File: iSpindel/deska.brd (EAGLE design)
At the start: 49.2 x 29.2 mm, 21 parts

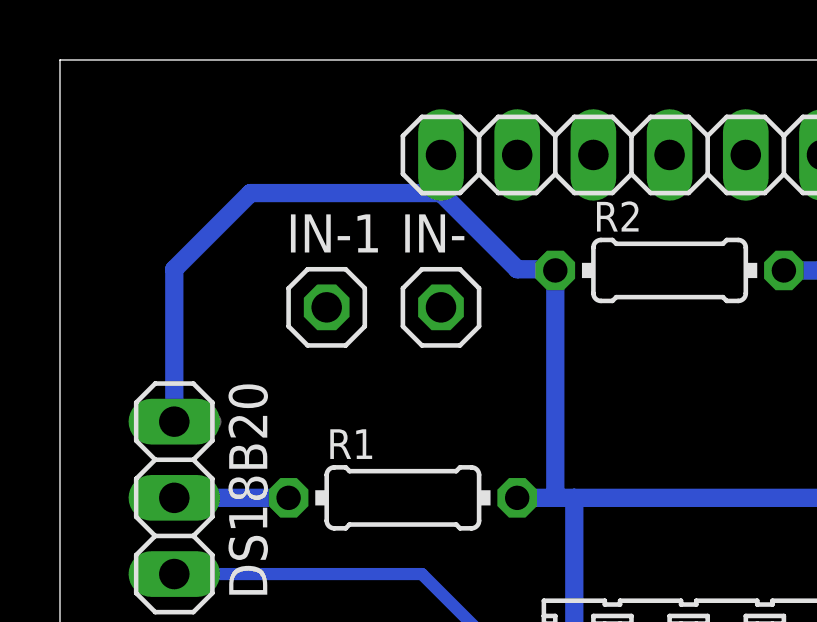
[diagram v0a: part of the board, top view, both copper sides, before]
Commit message: uprava desky
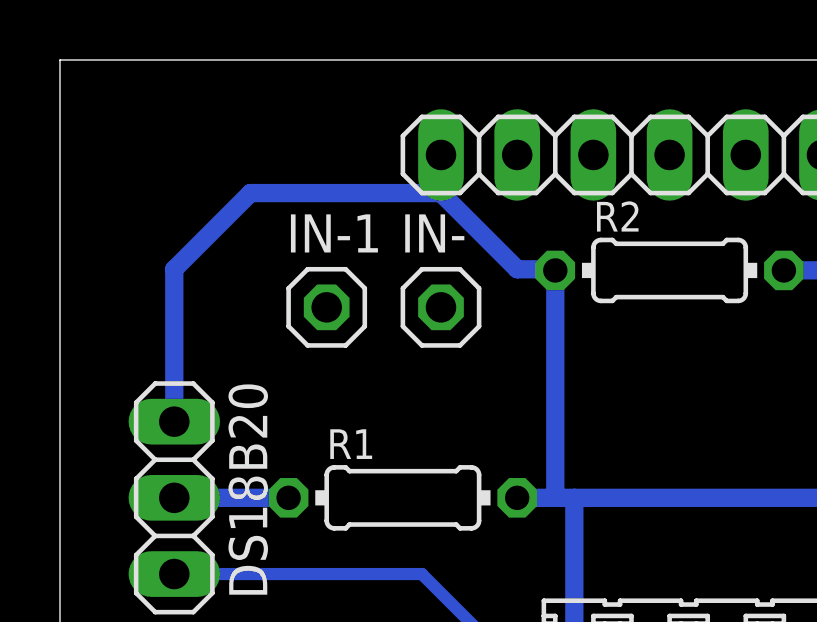
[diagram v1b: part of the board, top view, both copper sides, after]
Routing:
- net +3V3: track 65.3 -> 64.0 mm, vias 1 -> 0
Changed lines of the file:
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@@
 <?xml version="1.0" encoding="utf-8"?>
 <!DOCTYPE eagle SYSTEM "eagle.dtd">
-<eagle version="7.7.0">
+<eagle version="9.1.3">
 <drawing>
 <settings>
 <setting alwaysvectorfont="no"/>
+<setting keepoldvectorfont="yes"/>
 <setting verticaltext="up"/>
 </settings>
@@
 <param name="dpMaxLengthDifference" value="10mm"/>
 <param name="dpGapFactor" value="2.5"/>
-<param name="checkGrid" value="0"/>
 <param name="checkAngle" value="0"/>
 <param name="checkFont" value="1"/>
 <param name="checkRestrict" value="1"/>
+<param name="checkStop" value="0"/>
+<param name="checkValues" value="0"/>
+<param name="checkNames" value="1"/>
+<param name="checkWireStubs" value="1"/>
+<param name="checkPolygonWidth" value="0"/>
 <param name="useDiameter" value="13"/>
 <param name="maxErrors" value="50"/>
@@
 <element name="IN+3" library="pinhead" package="1X01" value="" x="38.1" y="12.065"/>
 <element name="SL1" library="con-amp-quick" package="05P" value="" x="22.225" y="13.335" rot="R180">
+<attribute name="MF" value="" x="22.225" y="13.335" size="1.778" layer="27" rot="R180" display="off"/>
 <attribute name="MPN" value="" x="22.225" y="13.335" size="1.778" layer="27" rot="R180" display="off"/>
+<attribute name="OC_FARNELL" value="unknown" x="22.225" y="13.335" size="1.778" layer="27" rot="R180" display="off"/>
 <attribute name="OC_NEWARK" value="unknown" x="22.225" y="13.335" size="1.778" layer="27" rot="R180" display="off"/>
-<attribute name="OC_FARNELL" value="unknown" x="22.225" y="13.335" size="1.778" layer="27" rot="R180" display="off"/>
-<attribute name="MF" value="" x="22.225" y="13.335" size="1.778" layer="27" rot="R180" display="off"/>
 </element>
 <element name="IN+4" library="pinhead" package="1X01" value="" x="38.1" y="24.765"/>
@@
 <contactref element="R1" pad="2"/>
 <wire x1="12.7" y1="30.48" x2="12.7" y2="29.21" width="0.6096" layer="16"/>
-<wire x1="12.7" y1="29.21" x2="15.24" y2="26.67" width="0.6096" layer="16"/>
-<wire x1="15.24" y1="26.67" x2="16.47" y2="26.67" width="0.6096" layer="16"/>
-<wire x1="16.47" y1="26.67" x2="16.51" y2="26.63" width="0.6096" layer="1"/>
-<wire x1="3.81" y1="21.59" x2="5.08" y2="21.59" width="0.6096" layer="1"/>
 <wire x1="12.7" y1="29.21" x2="6.35" y2="29.21" width="0.6096" layer="16"/>
 <wire x1="6.35" y1="29.21" x2="3.81" y2="26.67" width="0.6096" layer="16"/>
 <wire x1="3.81" y1="26.67" x2="3.81" y2="21.59" width="0.6096" layer="16"/>
-<via x="16.47" y="26.67" extent="1-16" drill="0.6" shape="square"/>
 <contactref element="SL1" pad="5"/>
 <wire x1="15.24" y1="19.05" x2="16.51" y2="19.05" width="0.6096" layer="16"/>
@@
 <wire x1="27.305" y1="19.05" x2="17.145" y2="19.05" width="0.6096" layer="16"/>
 <wire x1="29.21" y1="12.7" x2="30.48" y2="11.43" width="0.6096" layer="16"/>
+<wire x1="16.51" y1="26.63" x2="16.47" y2="26.67" width="0.6096" layer="16"/>
+<wire x1="16.47" y1="26.67" x2="15.24" y2="26.67" width="0.6096" layer="16"/>
+<wire x1="15.24" y1="26.67" x2="12.7" y2="29.21" width="0.6096" layer="16"/>
 </signal>
 <signal name="GND">
@@
 </signal>
 </signals>
+<mfgpreviewcolors>
+<mfgpreviewcolor name="soldermaskcolor" color="0xC8008000"/>
+<mfgpreviewcolor name="silkscreencolor" color="0xFFFEFEFE"/>
+<mfgpreviewcolor name="backgroundcolor" color="0xFF282828"/>
+<mfgpreviewcolor name="coppercolor" color="0xFFFFBF00"/>
+<mfgpreviewcolor name="substratecolor" color="0xFF786E46"/>
+</mfgpreviewcolors>
 </board>
 </drawing>
